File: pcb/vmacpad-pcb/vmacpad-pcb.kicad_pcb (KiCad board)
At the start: 2 copper layers, 156.1 x 117.1 mm, 30 parts, among them J1 TYPE-C-31-M12_13, SW1 SW_SPDT, U1 TPD4E05U06DQAR, U2 TXS0101DBVR, U3 STM32F401RCTx, Y1 16MHz

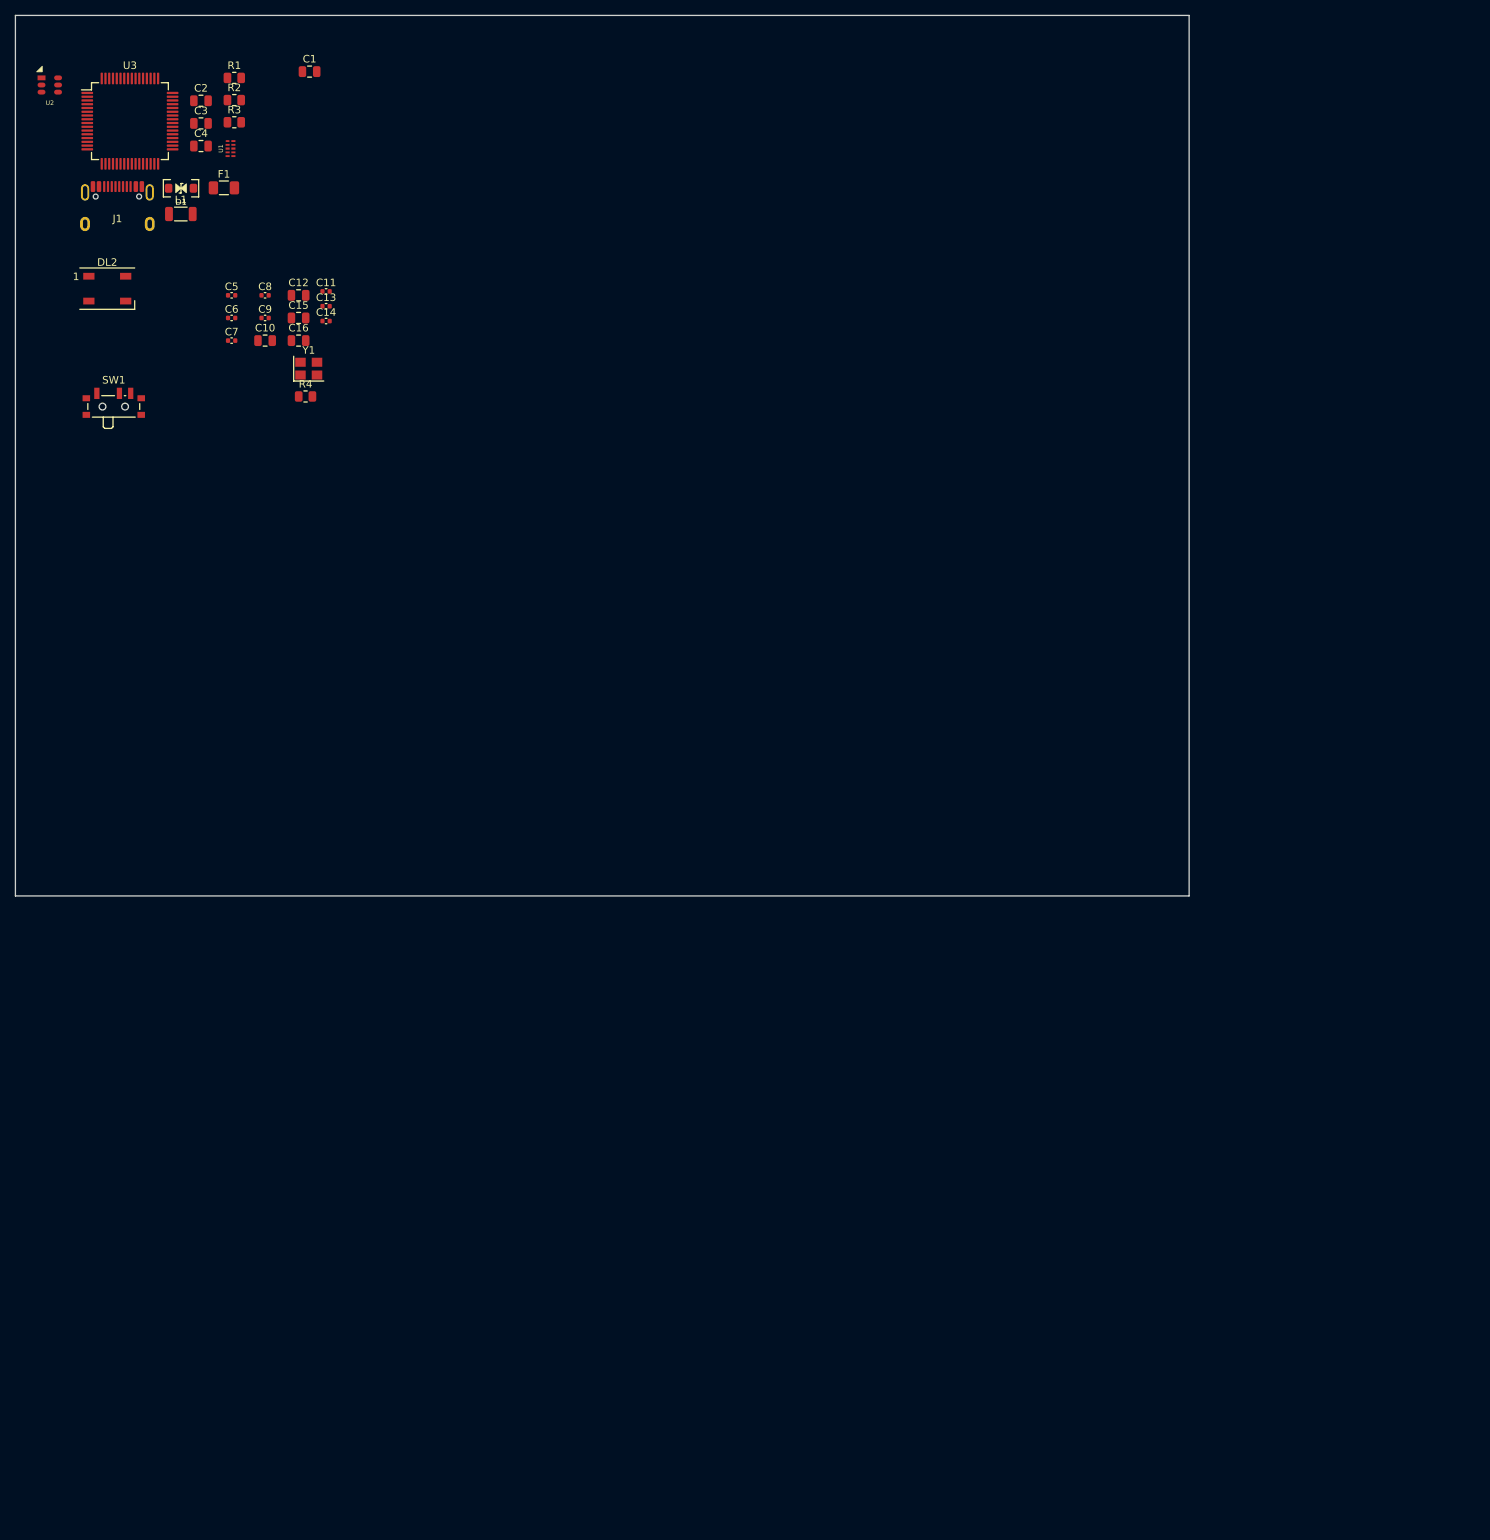
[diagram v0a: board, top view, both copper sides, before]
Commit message: Creating the PCB and additional parts
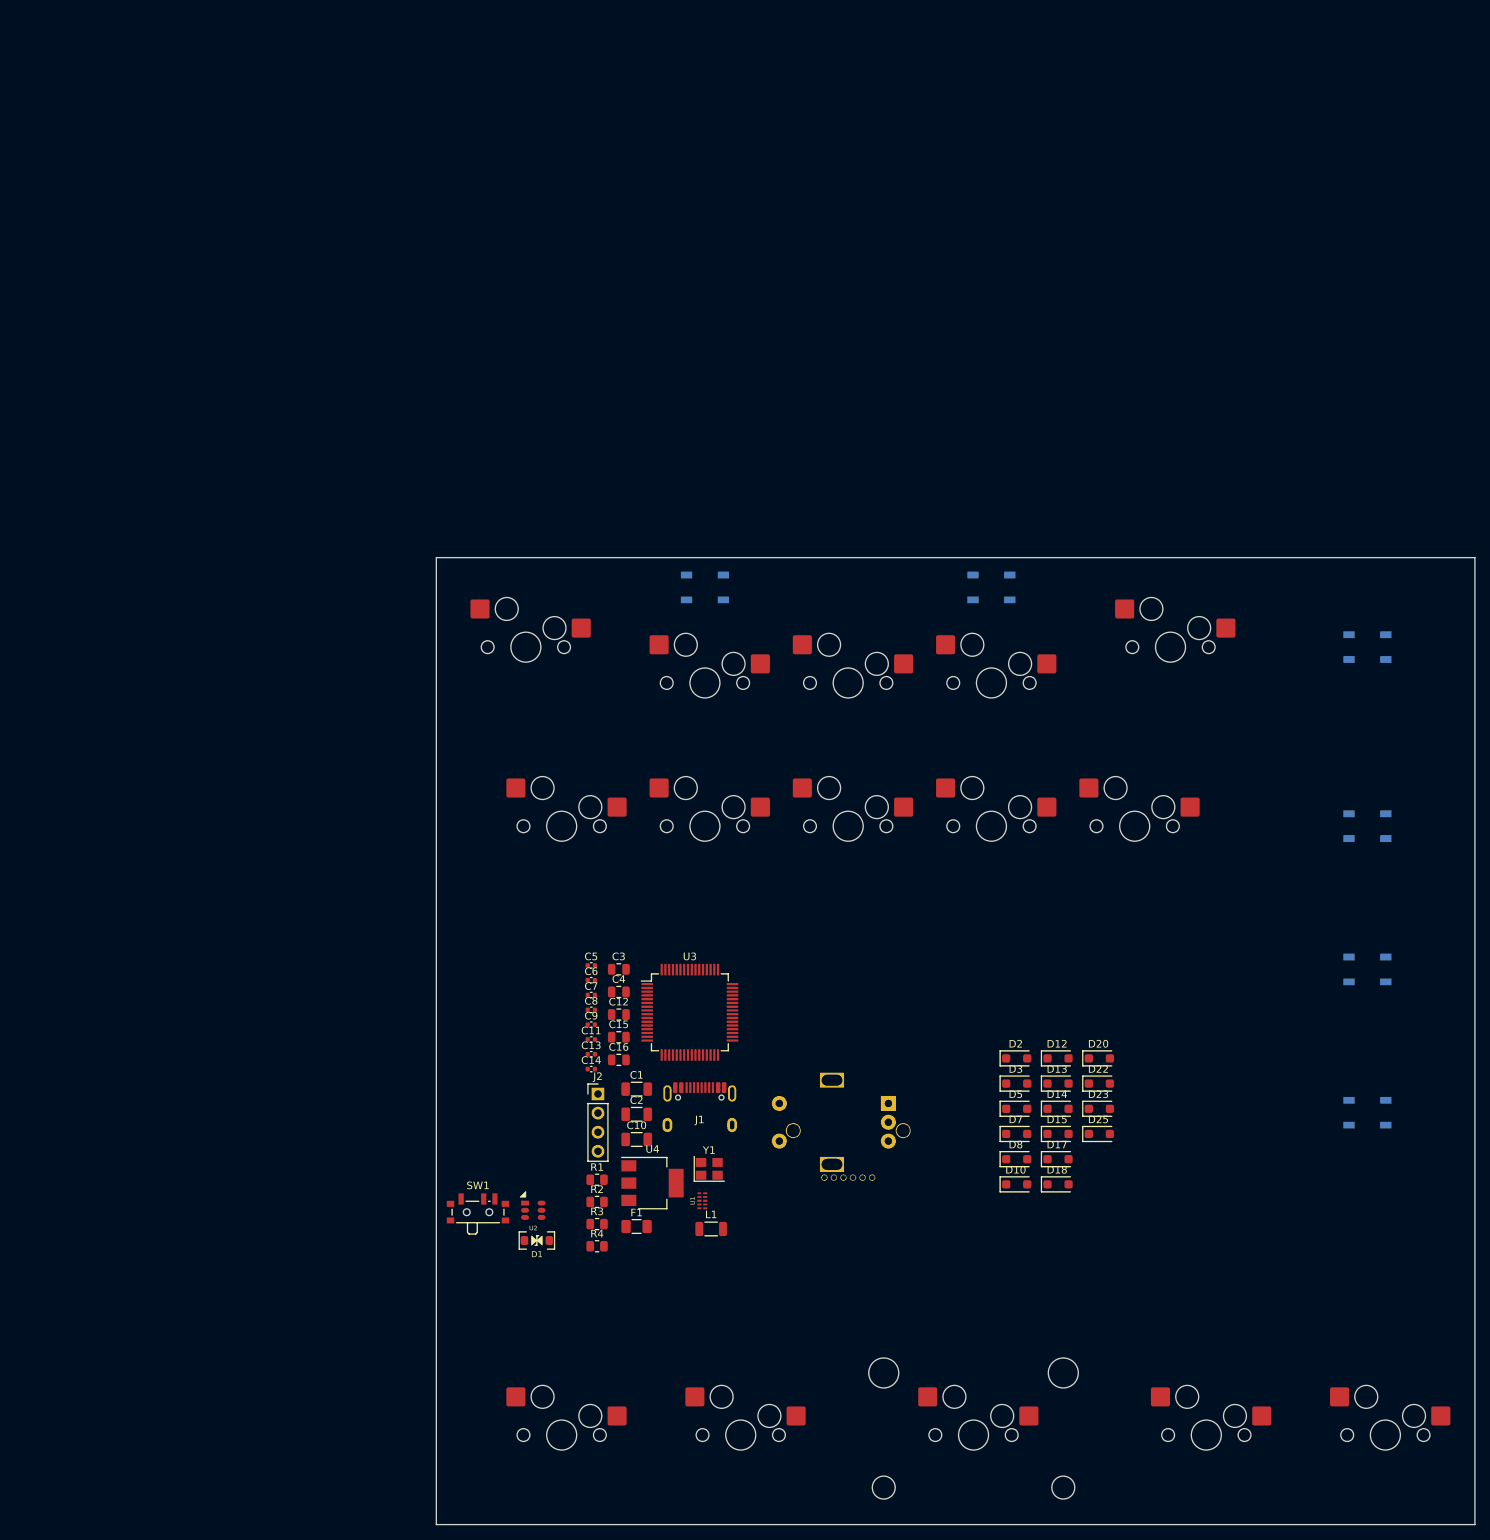
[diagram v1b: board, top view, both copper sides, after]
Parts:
- added D10: SM4007, Diode_SMD:D_SOD-123F, F.Cu at (165.3, 181.0)
- added D12: SM4007, Diode_SMD:D_SOD-123F, F.Cu at (170.8, 164.2)
- added D13: SM4007, Diode_SMD:D_SOD-123F, F.Cu at (170.8, 167.6)
- added D14: SM4007, Diode_SMD:D_SOD-123F, F.Cu at (170.8, 170.9)
- added D15: SM4007, Diode_SMD:D_SOD-123F, F.Cu at (170.8, 174.3)
- added D17: SM4007, Diode_SMD:D_SOD-123F, F.Cu at (170.8, 177.6)
- added D18: SM4007, Diode_SMD:D_SOD-123F, F.Cu at (170.8, 181.0)
- added D2: SM4007, Diode_SMD:D_SOD-123F, F.Cu at (165.3, 164.2)
- added D20: SM4007, Diode_SMD:D_SOD-123F, F.Cu at (176.3, 164.2)
- added D22: SM4007, Diode_SMD:D_SOD-123F, F.Cu at (176.3, 167.6)
- added D23: SM4007, Diode_SMD:D_SOD-123F, F.Cu at (176.3, 170.9)
- added D25: SM4007, Diode_SMD:D_SOD-123F, F.Cu at (176.3, 174.3)
- added D3: SM4007, Diode_SMD:D_SOD-123F, F.Cu at (165.3, 167.6)
- added D5: SM4007, Diode_SMD:D_SOD-123F, F.Cu at (165.3, 170.9)
- added D7: SM4007, Diode_SMD:D_SOD-123F, F.Cu at (165.3, 174.3)
- added D8: SM4007, Diode_SMD:D_SOD-123F, F.Cu at (165.3, 177.6)
- added DL1: WS2812B, LED_SMD:LED_WS2812B_PLCC4_5.0x5.0mm_P3.2mm, B.Cu at (211.9, 109.5)
- added DL3: WS2812B, LED_SMD:LED_WS2812B_PLCC4_5.0x5.0mm_P3.2mm, B.Cu at (211.9, 152.4)
- added DL4: WS2812B, LED_SMD:LED_WS2812B_PLCC4_5.0x5.0mm_P3.2mm, B.Cu at (211.9, 171.4)
- added DL5: WS2812B, LED_SMD:LED_WS2812B_PLCC4_5.0x5.0mm_P3.2mm, B.Cu at (161.9, 101.6)
- added DL6: WS2812B, LED_SMD:LED_WS2812B_PLCC4_5.0x5.0mm_P3.2mm, B.Cu at (123.8, 101.6)
- added J2: Conn_01x04_Pin, Connector_PinHeader_2.54mm:PinHeader_1x04_P2.54mm_Vertical, F.Cu at (109.6, 169.0)
- added K1: 1u, acheron_MXH:MX100H, F.Cu at (185.7, 109.5)
- added K10: 1u, acheron_MXH:MX100H, F.Cu at (142.9, 133.3)
- added K12: 2.25u, acheron_MXH:MX225HR, F.Cu at (159.5, 214.3)
- added K13: 1u, acheron_MXH:MX100H, F.Cu at (123.8, 114.3)
- added K14: 1u, acheron_MXH:MX100H, F.Cu at (123.8, 133.3)
- added K16: 1u, acheron_MXH:MX100H, F.Cu at (128.6, 214.3)
- added K17: 1u, acheron_MXH:MX100H, F.Cu at (100.0, 109.5)
- added K18: 1u, acheron_MXH:MX100H, F.Cu at (104.8, 133.3)
- added K2: 1u, acheron_MXH:MX100H, F.Cu at (181.0, 133.3)
- added K20: 1u, acheron_MXH:MX100H, F.Cu at (104.8, 214.3)
- added K4: 1u, acheron_MXH:MX100H, F.Cu at (214.3, 214.3)
- added K5: 1u, acheron_MXH:MX100H, F.Cu at (161.9, 114.3)
- added K6: 1u, acheron_MXH:MX100H, F.Cu at (161.9, 133.3)
- added K8: 1u, acheron_MXH:MX100H, F.Cu at (190.5, 214.3)
- added K9: 1u, acheron_MXH:MX100H, F.Cu at (142.9, 114.3)
- added SW2: Alps EM11, Rotary_Encoder:RotaryEncoder_Alps_EC11E-Switch_Vertical_H20mm, B.Cu at (148.2, 170.2)
- added SW3: BournsEM14, max_customs:BournsEM14, B.Cu at (142.9, 173.8)
- added U4: AMS1117-3.3, Package_TO_SOT_SMD:SOT-223-3_TabPin2, F.Cu at (116.9, 180.8)
- C1, C10, C2: footprint Capacitor_SMD:C_0805_2012Metric -> Capacitor_SMD:C_1206_3216Metric
- DL2: moved to B.Cu
- moved DL2 182.2 mm to (211.9, 133.3), turned to 180 degrees
- moved U2 162.9 mm to (101.0, 184.4)
- moved R1 154.3 mm to (109.5, 180.4)
- moved R2 154.3 mm to (109.5, 183.3)
- moved R3 154.3 mm to (109.5, 186.3)
- moved U1 153.3 mm to (123.5, 183.2)
- moved L1 152.3 mm to (124.7, 186.9)
- moved F1 148.6 mm to (114.7, 186.6)
- moved D1 147.7 mm to (101.5, 188.4)
- moved C2 146.7 mm to (114.8, 171.7)
- moved J1 142.7 mm to (123.1, 167.4)
- moved C1 142.1 mm to (114.8, 168.3)
- moved U3 140.0 mm to (121.8, 158.1)
- moved C3 125.5 mm to (112.4, 152.4)
- moved C4 125.5 mm to (112.4, 155.4)
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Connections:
- DL2 pad 2: unconnected-(DL2-DOUT-Pad2) -> Net-(DL2-DOUT)
- DL2 pad 4: RGB_5V -> Net-(DL1-DOUT)
- U3 pad 20: unconnected-(U3-PA4-Pad20) -> COL0
- U3 pad 21: unconnected-(U3-PA5-Pad21) -> COL1
- U3 pad 22: unconnected-(U3-PA6-Pad22) -> COL2
- U3 pad 23: unconnected-(U3-PA7-Pad23) -> COL3
- U3 pad 24: unconnected-(U3-PC4-Pad24) -> ENC_PADA
- U3 pad 25: unconnected-(U3-PC5-Pad25) -> ENC_PADB
- U3 pad 26: unconnected-(U3-PB0-Pad26) -> ROW0
- U3 pad 27: unconnected-(U3-PB1-Pad27) -> ROW1
- U3 pad 41: unconnected-(U3-PA8-Pad41) -> COL4
- U3 pad 46: SWDIO -> /SWDIO
- U3 pad 49: SWCLK -> /SWCLK
- U3 pad 55: unconnected-(U3-PB3-Pad55) -> ROW2
- U3 pad 56: unconnected-(U3-PB4-Pad56) -> ROW3
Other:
- board size 156.1 x 117.1 mm -> 138.1 x 128.6 mm
